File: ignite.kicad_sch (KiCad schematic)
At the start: 8 parts

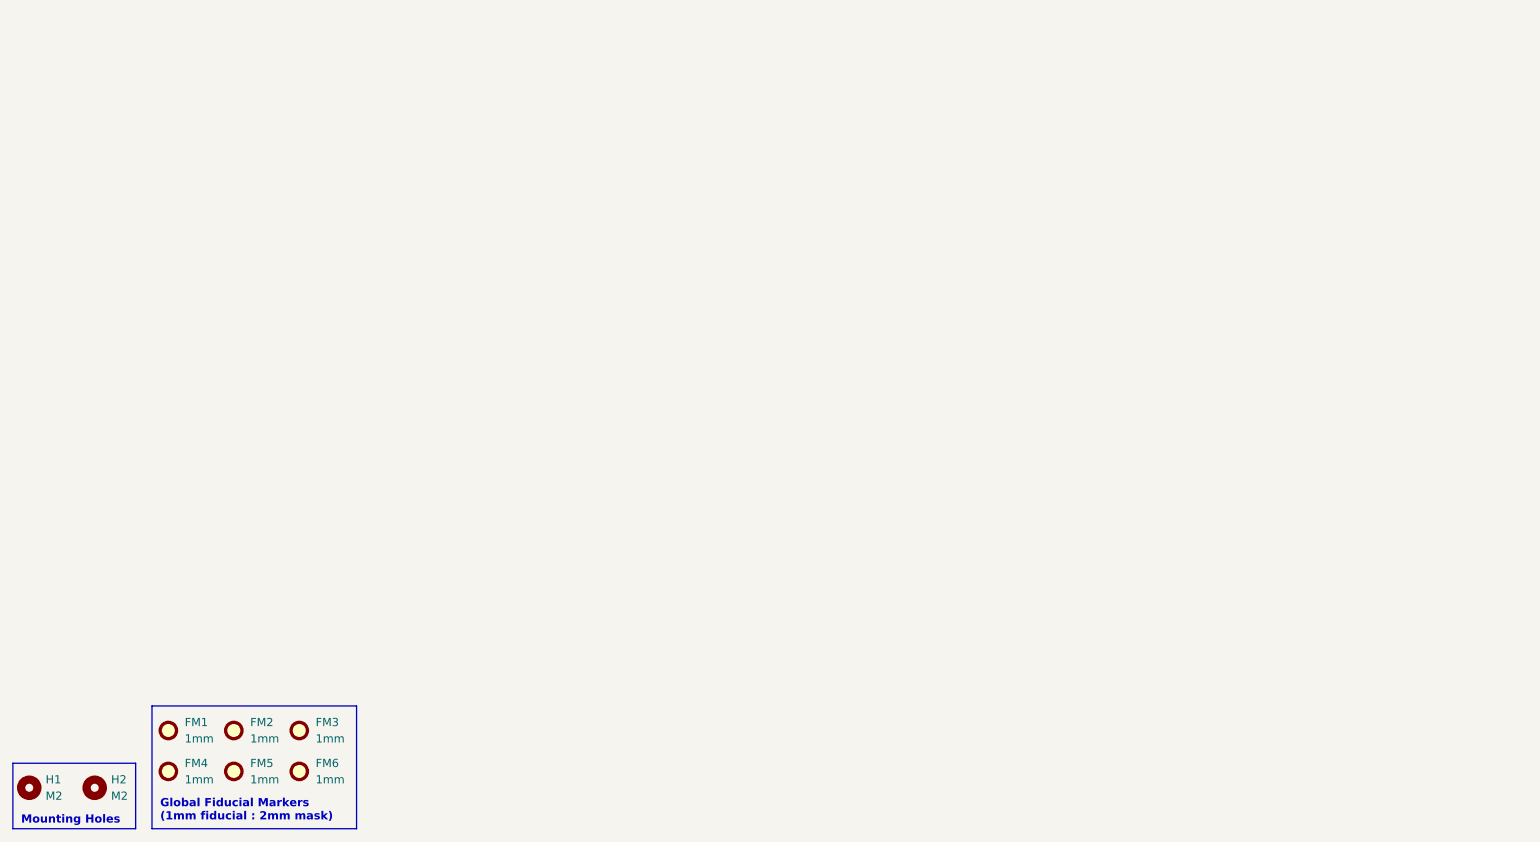
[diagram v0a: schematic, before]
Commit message: Add WIP schematic
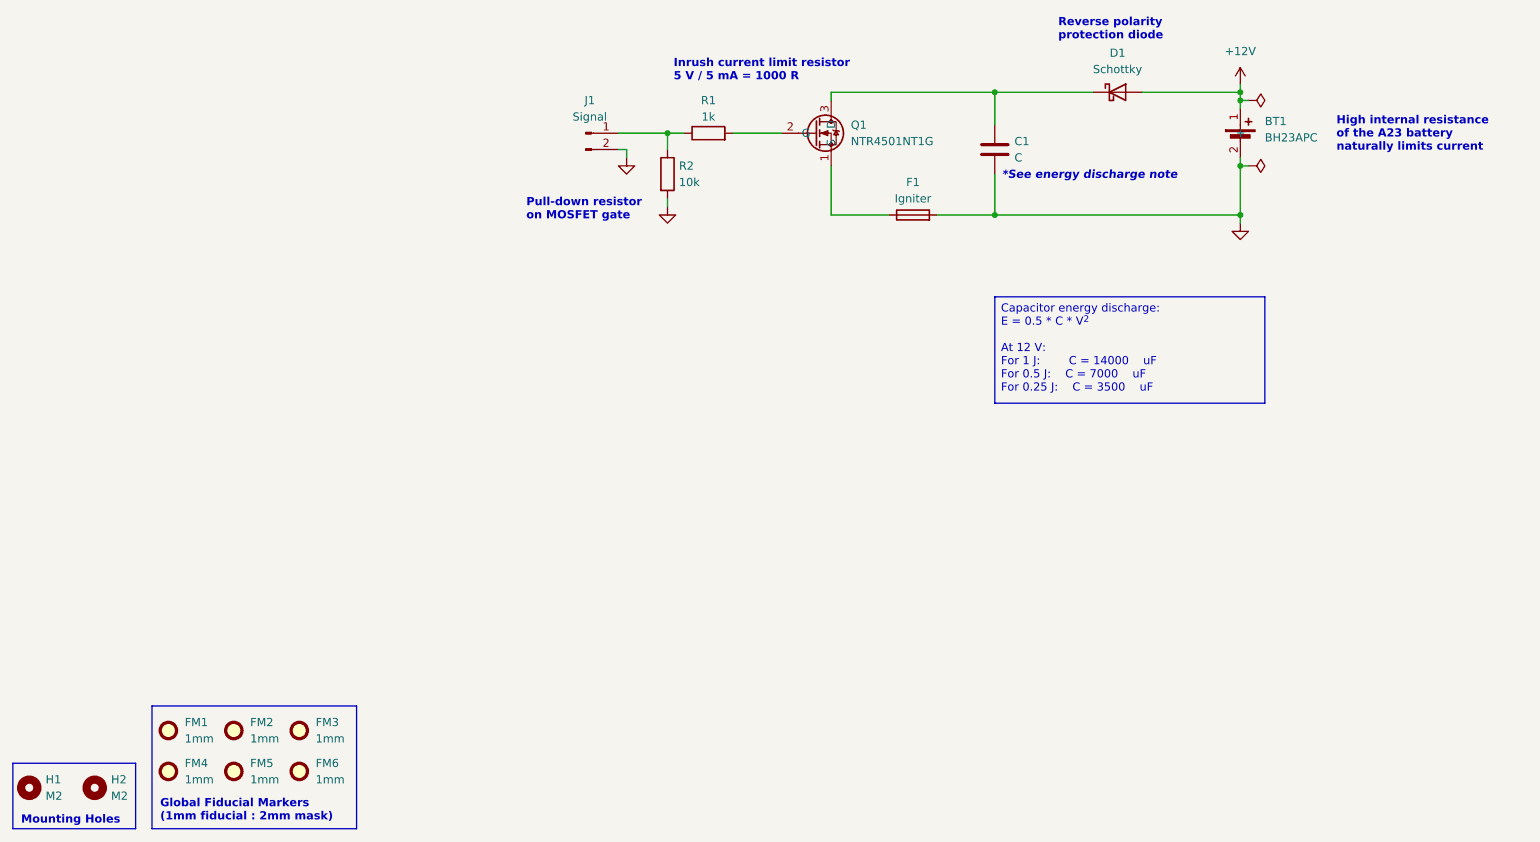
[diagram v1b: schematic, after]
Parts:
- added BT1: BH23APC, bh23:bh23apc, symbol bh23:bh23apc
- added C1: C, symbol Device:C
- added D1: Schottky, symbol Device:D_Schottky
- added F1: Igniter, symbol Device:Fuse
- added J1: Signal, symbol Connector:Conn_01x02_Pin
- added Q1: NTR4501NT1G, Package_TO_SOT_SMD:SOT-23-3, symbol ntr4501nt1g:ntr4501nt1g
- added R1: 1k, symbol Device:R
- added R2: 10k, symbol Device:R
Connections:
- new net: J1.1 (Pin_1), R1.1, R2.1
- new net: Q1.2 (G), R1.2
- new net: C1.1, D1.1 (K), Q1.3 (D)
- new net: F1.1, Q1.1 (S)
- new net +12V: BT1.1 (+), D1.2 (A)
- new net GND: BT1.2 (-), C1.2, F1.2, J1.2 (Pin_2), R2.2
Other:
- note added: "*See energy discharge note"
